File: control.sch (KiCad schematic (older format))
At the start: 19 parts, among them P601 Programmer, SW601 SW_Push, U601 ATMEGA328P-PU, Y601 16 MHz

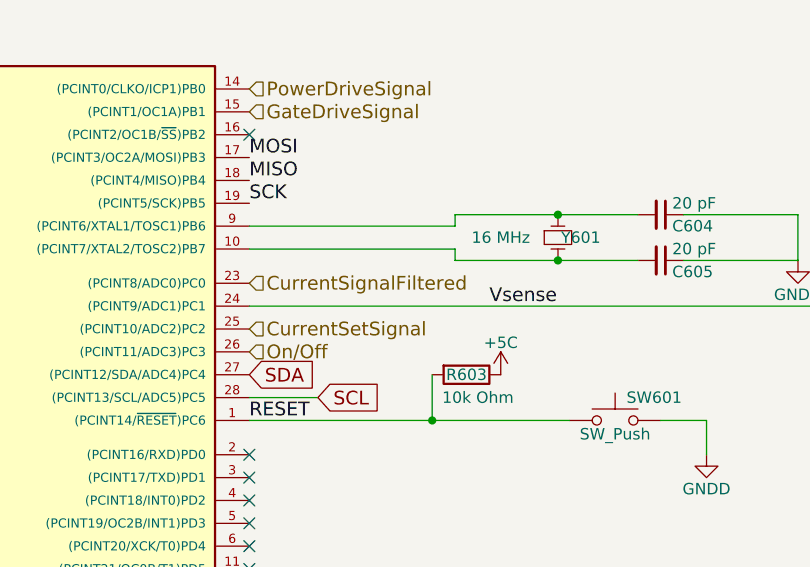
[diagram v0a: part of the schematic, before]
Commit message: New amplifiers, fuse and general mayhem
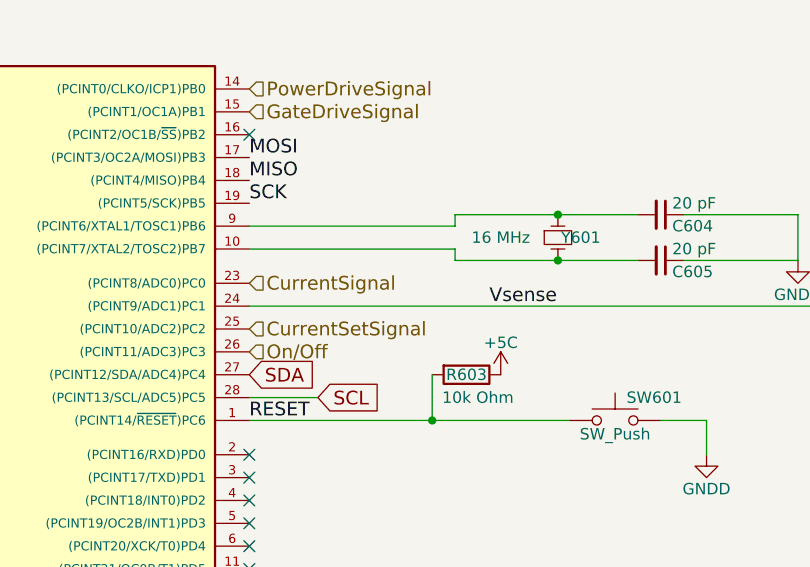
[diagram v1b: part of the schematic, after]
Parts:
- C601, C602, C603, C604, C605, C607: footprint Capacitors_SMD:C_0603 -> axel:C_0603_CustomText
- C606: footprint Capacitors_SMD:C_0805 -> axel:C_0805_CustomText
- R601, R602, R603, R604, R605, R606, R607: footprint Resistors_SMD:R_0603 -> axel:C_0603_CustomText
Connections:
- net CurrentSignalFiltered renamed CurrentSignal
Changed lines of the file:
@@
 RESET
 $Comp
-L +5C #PWR028
+L +5C #PWR027
 U 1 1 58E658EA
 P 4150 950
-F 0 "#PWR028" H 4150 800 50  0001 C CNN
+F 0 "#PWR027" H 4150 800 50  0001 C CNN
 F 1 "+5C" H 4150 1090 50  0000 C CNN
 F 2 "" H 4150 950 50  0000 C CNN
@@
 $EndComp
 $Comp
-L +5C #PWR029
+L +5C #PWR028
 U 1 1 58E658EB
 P 2100 1800
-F 0 "#PWR029" H 2100 1650 50  0001 C CNN
+F 0 "#PWR028" H 2100 1650 50  0001 C CNN
 F 1 "+5C" H 2100 1940 50  0000 C CNN
 F 2 "" H 2100 1800 50  0000 C CNN
@@
 F 0 "C602" H 2560 2120 50  0000 L CNN
 F 1 "100 nF" H 2560 1970 50  0000 L CNN
-F 2 "Capacitors_SMD:C_0603" H 2550 2050 50  0001 C CNN
+F 2 "axel:C_0603_CustomText" H 2550 2050 50  0001 C CNN
 F 3 "" H 2550 2050 50  0000 C CNN
 	1    2550 2050
@@
 $EndComp
 $Comp
-L GNDD #PWR030
+L GNDD #PWR029
 U 1 1 58E658EE
 P 4150 1150
-F 0 "#PWR030" H 4150 900 50  0001 C CNN
+F 0 "#PWR029" H 4150 900 50  0001 C CNN
 F 1 "GNDD" H 4150 1000 50  0000 C CNN
 F 2 "" H 4150 1150 50  0000 C CNN
@@
 $EndComp
 $Comp
-L GNDD #PWR031
+L GNDD #PWR030
 U 1 1 58E658EF
 P 2550 2150
-F 0 "#PWR031" H 2550 1900 50  0001 C CNN
+F 0 "#PWR030" H 2550 1900 50  0001 C CNN
 F 1 "GNDD" H 2550 2000 50  0000 C CNN
 F 2 "" H 2550 2150 50  0000 C CNN
@@
 $EndComp
 $Comp
-L GNDD #PWR032
+L GNDD #PWR031
 U 1 1 58E658F2
 P 2950 4350
-F 0 "#PWR032" H 2950 4100 50  0001 C CNN
+F 0 "#PWR031" H 2950 4100 50  0001 C CNN
 F 1 "GNDD" H 2950 4200 50  0000 C CNN
 F 2 "" H 2950 4350 50  0000 C CNN
@@
 F 0 "C604" V 6700 2650 50  0000 L CNN
 F 1 "20 pF" V 6600 2650 50  0000 L CNN
-F 2 "Capacitors_SMD:C_0603" H 6650 2600 50  0001 C CNN
+F 2 "axel:C_0603_CustomText" H 6650 2600 50  0001 C CNN
 F 3 "" H 6650 2600 50  0000 C CNN
 	1    6650 2600
@@
 F 0 "C605" V 6700 2850 50  0000 L CNN
 F 1 "20 pF" V 6600 2850 50  0000 L CNN
-F 2 "Capacitors_SMD:C_0603" H 6650 2800 50  0001 C CNN
+F 2 "axel:C_0603_CustomText" H 6650 2800 50  0001 C CNN
 F 3 "" H 6650 2800 50  0000 C CNN
 	1    6650 2800
@@
 Connection ~ 6200 2600
 $Comp
-L GNDD #PWR033
+L GNDD #PWR032
 U 1 1 58E65F74
 P 7250 2800
-F 0 "#PWR033" H 7250 2550 50  0001 C CNN
+F 0 "#PWR032" H 7250 2550 50  0001 C CNN
 F 1 "GNDD" H 7250 2650 50  0000 C CNN
 F 2 "" H 7250 2800 50  0000 C CNN
@@
 F 0 "R601" V 2350 2050 50  0000 C CNN
 F 1 "100 Ohm" V 2450 2050 50  0000 C CNN
-F 2 "Resistors_SMD:R_0603" V 2280 2050 50  0001 C CNN
+F 2 "axel:C_0603_CustomText" V 2280 2050 50  0001 C CNN
 F 3 "" H 2350 2050 50  0000 C CNN
 	1    2350 2050
@@
 F 0 "C601" H 2360 2870 50  0000 L CNN
 F 1 "100 nF" H 2360 2720 50  0000 L CNN
-F 2 "Capacitors_SMD:C_0603" H 2350 2800 50  0001 C CNN
+F 2 "axel:C_0603_CustomText" H 2350 2800 50  0001 C CNN
 F 3 "" H 2350 2800 50  0000 C CNN
 	1    2350 2800
@@
 F 0 "C603" H 2760 2870 50  0000 L CNN
 F 1 "100 nF" H 2800 2750 50  0000 L CNN
-F 2 "Capacitors_SMD:C_0603" H 2750 2800 50  0001 C CNN
+F 2 "axel:C_0603_CustomText" H 2750 2800 50  0001 C CNN
 F 3 "" H 2750 2800 50  0000 C CNN
 	1    2750 2800
@@
 F 0 "R603" V 5800 3300 50  0000 C CNN
 F 1 "10k Ohm" V 5900 3350 50  0000 C CNN
-F 2 "Resistors_SMD:R_0603" V 5730 3300 50  0001 C CNN
+F 2 "axel:C_0603_CustomText" V 5730 3300 50  0001 C CNN
 F 3 "" H 5800 3300 50  0000 C CNN
 	1    5800 3300
@@
 $EndComp
 $Comp
-L +5C #PWR034
+L +5C #PWR033
 U 1 1 58E666D5
 P 5950 3300
-F 0 "#PWR034" H 5950 3150 50  0001 C CNN
+F 0 "#PWR033" H 5950 3150 50  0001 C CNN
 F 1 "+5C" H 5950 3440 50  0000 C CNN
 F 2 "" H 5950 3300 50  0000 C CNN
@@
 	4850 3500 6250 3500
 $Comp
-L GNDD #PWR035
+L GNDD #PWR034
 U 1 1 58E673C7
 P 6850 3650
-F 0 "#PWR035" H 6850 3400 50  0001 C CNN
+F 0 "#PWR034" H 6850 3400 50  0001 C CNN
 F 1 "GNDD" H 6850 3500 50  0000 C CNN
 F 2 "" H 6850 3650 50  0000 C CNN
@@
 	5650 3300 5650 3500
 $Comp
-L GNDREF #PWR036
+L GNDREF #PWR035
 U 1 1 58E7A421
 P 2650 4350
-F 0 "#PWR036" H 2650 4100 50  0001 C CNN
+F 0 "#PWR035" H 2650 4100 50  0001 C CNN
 F 1 "GNDREF" H 2650 4200 50  0000 C CNN
 F 2 "" H 2650 4350 50  0000 C CNN
@@
 	2650 4250 2950 4250
 $Comp
-L VCC #PWR037
+L VCC #PWR036
 U 1 1 58E7C132
 P 8500 2050
-F 0 "#PWR037" H 8500 1900 50  0001 C CNN
+F 0 "#PWR036" H 8500 1900 50  0001 C CNN
 F 1 "VCC" H 8500 2200 50  0000 C CNN
 F 2 "" H 8500 2050 50  0000 C CNN
@@
 F 0 "C607" H 8510 2820 50  0000 L CNN
 F 1 "100 nF" H 8510 2670 50  0000 L CNN
-F 2 "Capacitors_SMD:C_0603" H 8500 2750 50  0001 C CNN
+F 2 "axel:C_0603_CustomText" H 8500 2750 50  0001 C CNN
 F 3 "" H 8500 2750 50  0000 C CNN
 	1    8500 2750
@@
 F 0 "C606" H 8160 2820 50  0000 L CNN
 F 1 "1 uF" H 8160 2670 50  0000 L CNN
-F 2 "Capacitors_SMD:C_0805" H 8150 2750 50  0001 C CNN
+F 2 "axel:C_0805_CustomText" H 8150 2750 50  0001 C CNN
 F 3 "" H 8150 2750 50  0000 C CNN
 	1    8150 2750
@@
 F 0 "R606" V 7750 2750 50  0000 C CNN
 F 1 "4.7 kOhm" V 7650 2750 50  0000 C CNN
-F 2 "Resistors_SMD:R_0603" V 7680 2750 50  0001 C CNN
+F 2 "axel:C_0603_CustomText" V 7680 2750 50  0001 C CNN
 F 3 "" H 7750 2750 50  0000 C CNN
 	1    7750 2750
@@
 F 0 "R607" V 7750 3250 50  0000 C CNN
 F 1 "4.7 kOhm" V 7650 3250 50  0000 C CNN
-F 2 "Resistors_SMD:R_0603" V 7680 3250 50  0001 C CNN
+F 2 "axel:C_0603_CustomText" V 7680 3250 50  0001 C CNN
 F 3 "" H 7750 3250 50  0000 C CNN
 	1    7750 3250
@@
 Connection ~ 7750 3000
 $Comp
-L GNDREF #PWR038
+L GNDREF #PWR037
 U 1 1 58E7CFC1
 P 7750 3650
-F 0 "#PWR038" H 7750 3400 50  0001 C CNN
+F 0 "#PWR037" H 7750 3400 50  0001 C CNN
 F 1 "GNDREF" H 7750 3500 50  0000 C CNN
 F 2 "" H 7750 3650 50  0000 C CNN
@@
 $EndComp
 $Comp
-L GNDREF #PWR039
+L GNDREF #PWR038
 U 1 1 58E7CFFC
 P 8500 3650
-F 0 "#PWR039" H 8500 3400 50  0001 C CNN
+F 0 "#PWR038" H 8500 3400 50  0001 C CNN
 F 1 "GNDREF" H 8500 3500 50  0000 C CNN
 F 2 "" H 8500 3650 50  0000 C CNN
@@
 F 0 "R602" V 2750 2050 50  0000 C CNN
 F 1 "100 Ohm" V 2850 2050 50  0000 C CNN
-F 2 "Resistors_SMD:R_0603" V 2680 2050 50  0001 C CNN
+F 2 "axel:C_0603_CustomText" V 2680 2050 50  0001 C CNN
 F 3 "" H 2750 2050 50  0000 C CNN
 	1    2750 2050
@@
 	2750 2200 2750 2700
 $Comp
-L GNDREF #PWR040
+L GNDREF #PWR039
 U 1 1 58E7FF6D
 P 2350 2950
-F 0 "#PWR040" H 2350 2700 50  0001 C CNN
+F 0 "#PWR039" H 2350 2700 50  0001 C CNN
 F 1 "GNDREF" H 2350 2800 50  0000 C CNN
 F 2 "" H 2350 2950 50  0000 C CNN
@@
 $EndComp
 $Comp
-L GNDREF #PWR041
+L GNDREF #PWR040
 U 1 1 58E7FFB2
 P 2750 2950
-F 0 "#PWR041" H 2750 2700 50  0001 C CNN
+F 0 "#PWR040" H 2750 2700 50  0001 C CNN
 F 1 "GNDREF" H 2750 2800 50  0000 C CNN
 F 2 "" H 2750 2950 50  0000 C CNN
@@
 F 0 "R604" V 5980 5450 50  0000 C CNN
 F 1 "4.7k" V 5900 5450 50  0000 C CNN
-F 2 "Resistors_SMD:R_0603" V 5830 5450 50  0001 C CNN
+F 2 "axel:C_0603_CustomText" V 5830 5450 50  0001 C CNN
 F 3 "" H 5900 5450 50  0000 C CNN
 	1    5900 5450
@@
 F 0 "R605" V 6180 4800 50  0000 C CNN
 F 1 "4.7k" V 6100 4800 50  0000 C CNN
-F 2 "Resistors_SMD:R_0603" V 6030 4800 50  0001 C CNN
+F 2 "axel:C_0603_CustomText" V 6030 4800 50  0001 C CNN
 F 3 "" H 6100 4800 50  0000 C CNN
 	1    6100 4800
@@
 	5900 5700 5900 5600
 $Comp
-L +5C #PWR042
+L +5C #PWR041
 U 1 1 58F9C5AB
 P 5900 4500
-F 0 "#PWR042" H 5900 4350 50  0001 C CNN
+F 0 "#PWR041" H 5900 4350 50  0001 C CNN
 F 1 "+5C" H 5900 4640 50  0000 C CNN
 F 2 "" H 5900 4500 50  0000 C CNN
@@
 Connection ~ 5900 4550
 Text HLabel 4850 2900 2    60   Input ~ 0
-CurrentSignalFiltered
+CurrentSignal
 $Comp
 L ATMEGA328P-PU U601
